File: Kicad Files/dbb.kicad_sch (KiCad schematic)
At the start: 13 parts, among them U18 74HC245, U19 MAX7375AXR105, U20 74LS161, U21 74LS139, U21 SST39SF020, U23 HDSP-A151, U24 HDSP-A151, U25 HDSP-A151, U26 HDSP-A151

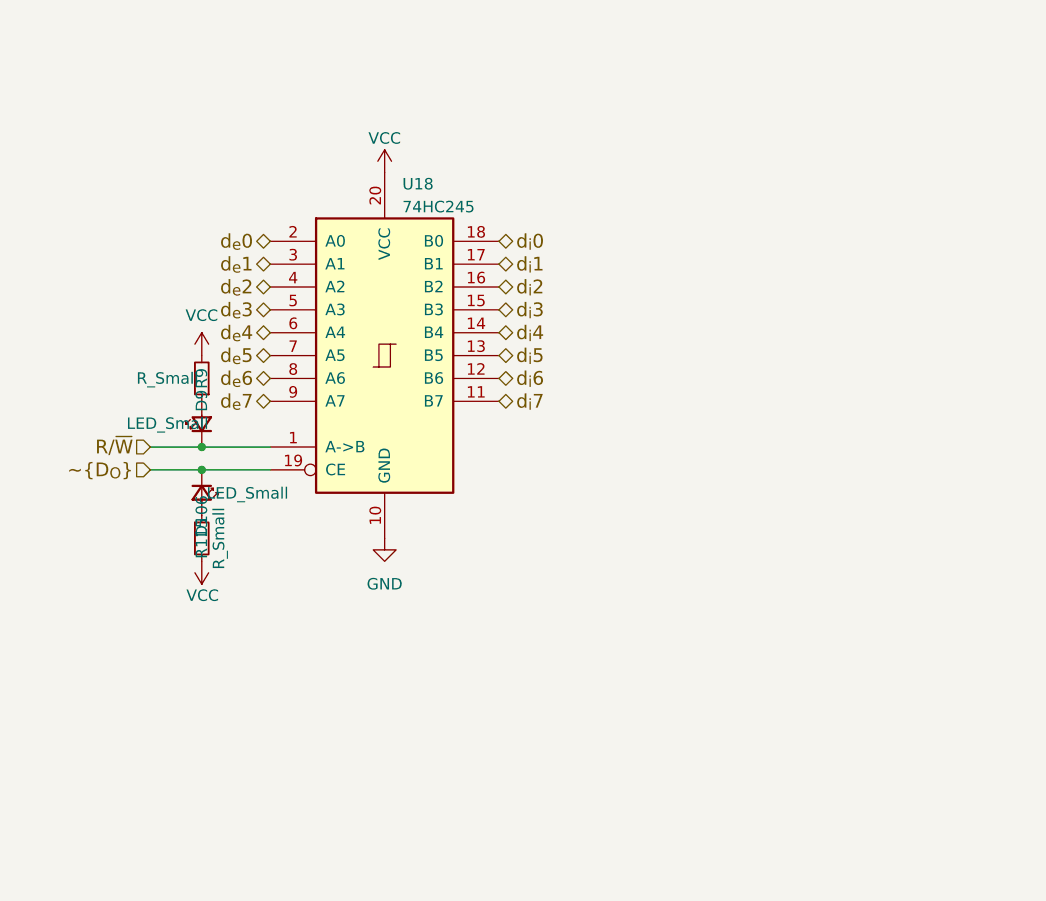
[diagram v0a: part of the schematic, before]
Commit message: rethink alu
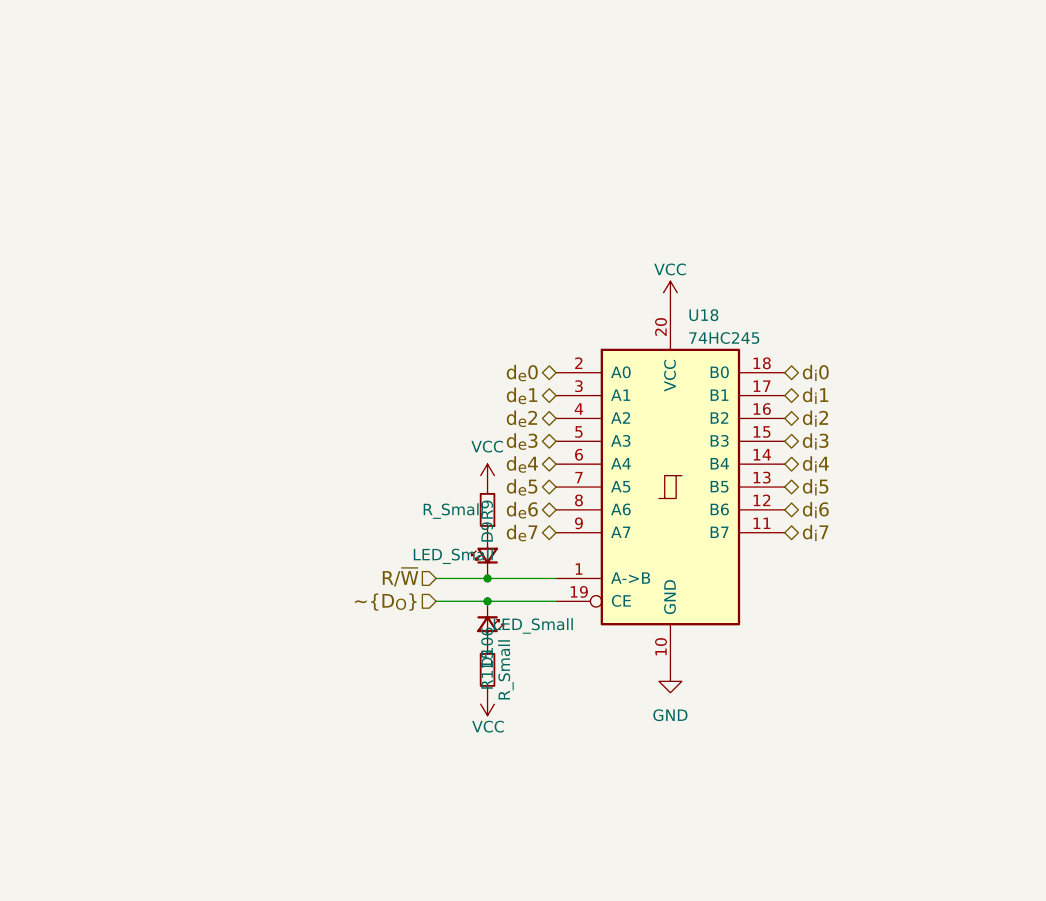
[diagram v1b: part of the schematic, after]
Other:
- moved on the sheet: D106, D9, R115, R9, U18
